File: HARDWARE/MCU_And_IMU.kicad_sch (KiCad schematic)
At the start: 16 parts, among them U2 STM32G431KBTx, Y1 Crystal_GND24

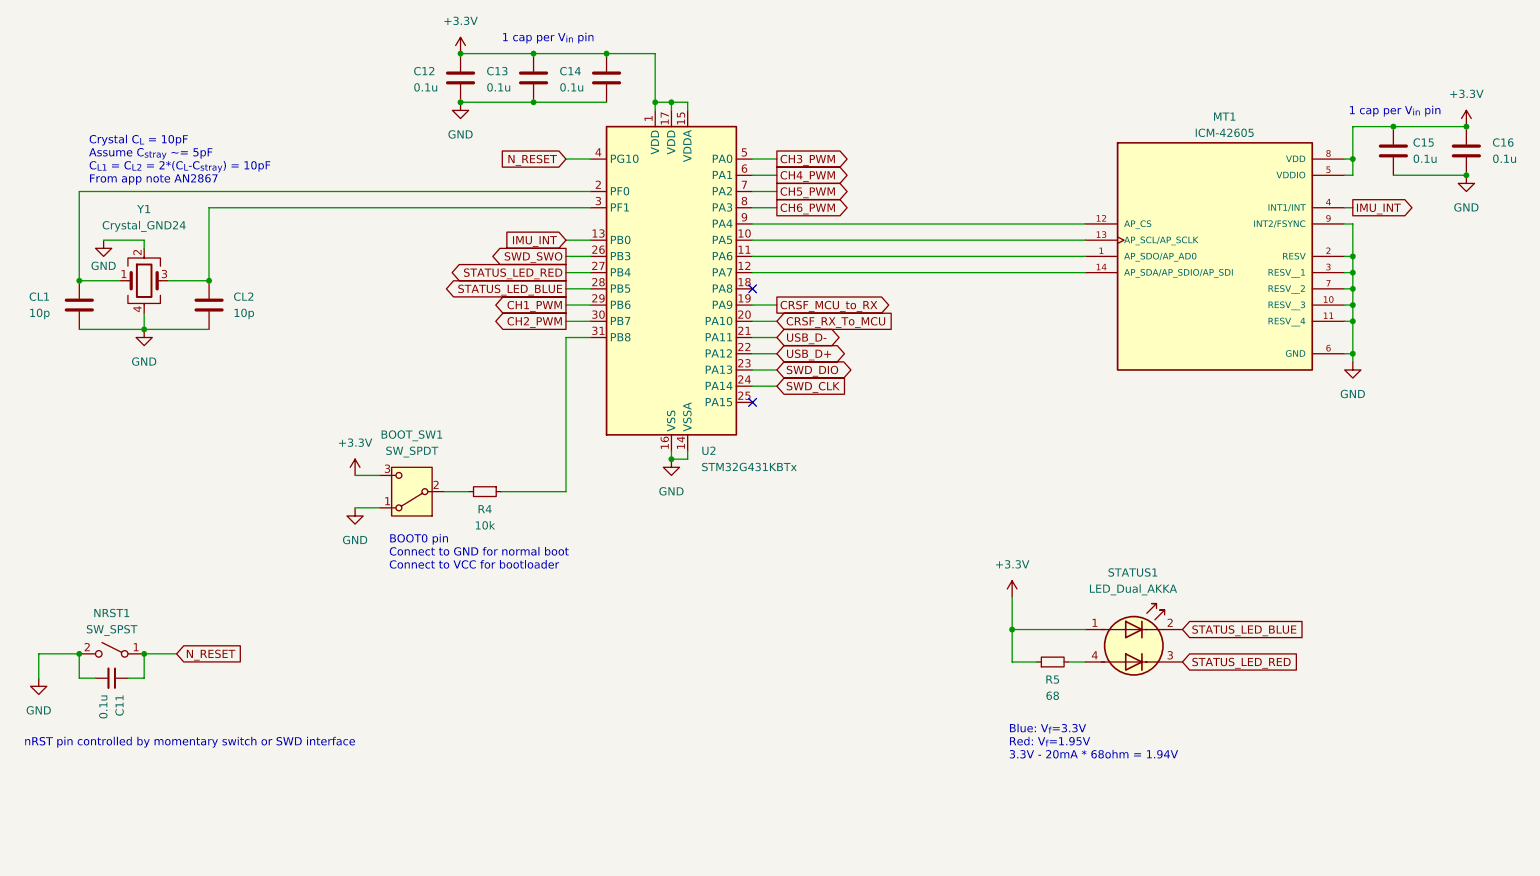
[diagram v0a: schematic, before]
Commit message: Update footprints and add all PNs
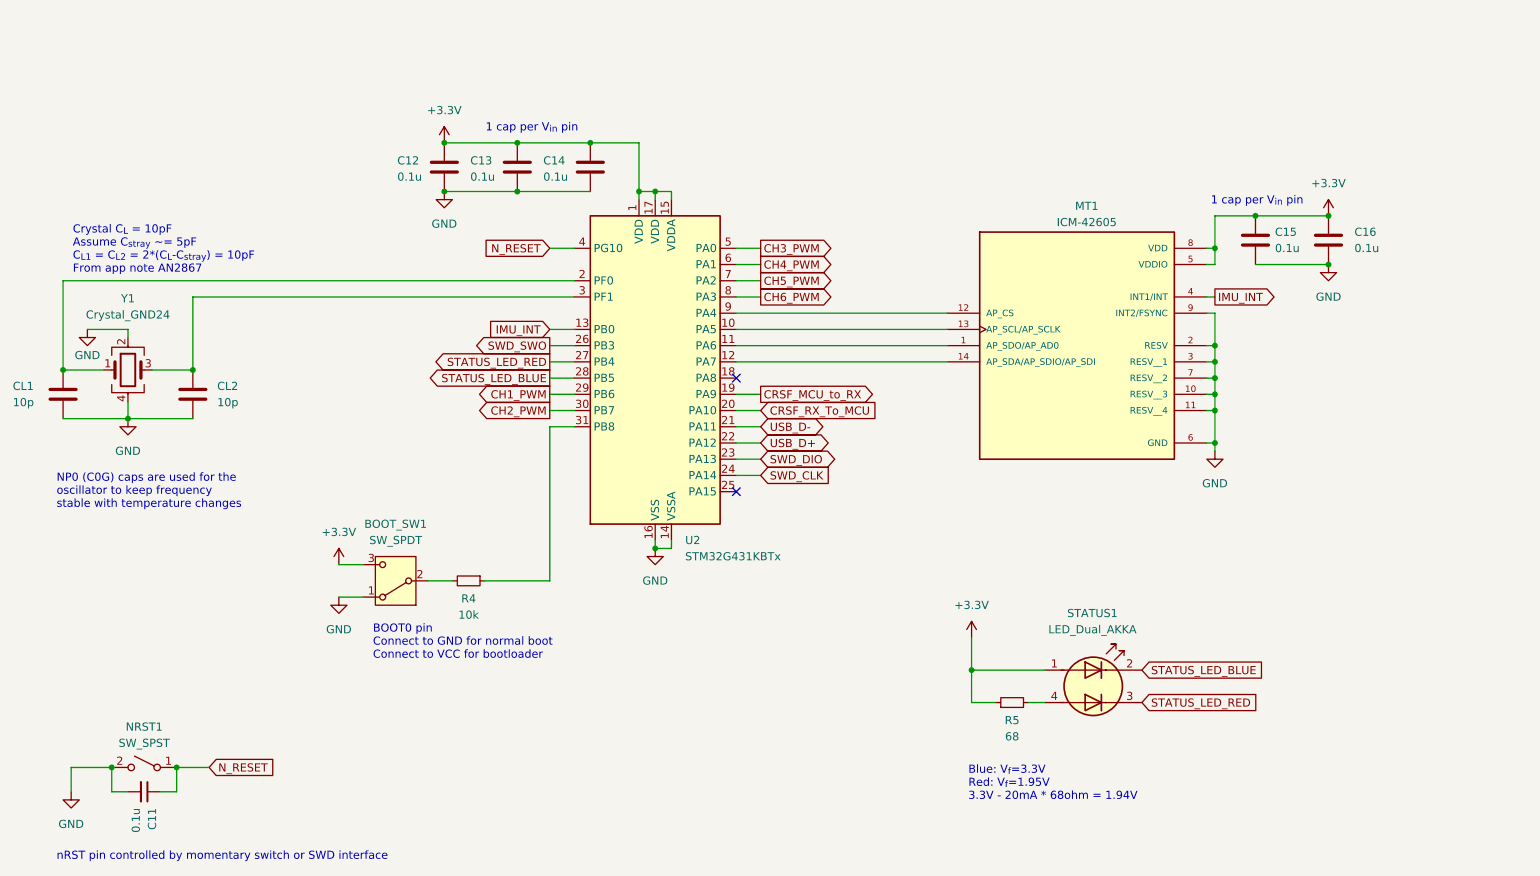
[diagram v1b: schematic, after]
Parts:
- BOOT_SW1: footprint (none) -> Button_Switch_THT_Custom:SW_SLW-883935-2A-D
- C11, C12, C13, C14, C15, C16: Part Number (none) -> 311-1341-2-ND
- CL1, CL2: Part Number (none) -> 311-3908-2-ND
- NRST1: footprint (none) -> Button_Switch_SMD_Custom:SW_Tactile_SPST_PTS636SK25FSMTRLFS; Part Number 108-PTS636SM43SMTRLFSTR-ND -> CKN12330-2-ND
- R4: Part Number (none) -> 311-10.0KHRTR-ND
- R5: Part Number (none) -> 311-68.0HRTR-ND
- STATUS1: footprint (none) -> LED_SMD_Custom:LED_APHBM2012QBDSURKC
- Y1: footprint (none) -> Crystal_Custom:XTAL_ECS-80-10-30B-CKM-TR
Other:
- note added: "NP0 (C0G) caps are used for the oscillator to keep frequency stable with temperature changes"
- moved on the sheet: BOOT_SW1, C11, C12, C13, C14, C15, C16, CL1, CL2, MT1, NRST1, R4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
